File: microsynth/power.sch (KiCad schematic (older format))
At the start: 4 parts, among them J2 AudioJack2, J3 AudioJack2, J4 AudioJack2, J5 AudioJack2

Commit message: Footprints 2
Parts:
- J2, J3, J4, J5: footprint (none) -> Connector_Audio:Jack_3.5mm_QingPu_WQP-PJ398SM_Vertical_CircularHoles
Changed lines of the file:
@@
 F 0 "J2" H 3820 2170 50  0000 R CNN
 F 1 "AudioJack2" H 3820 2079 50  0000 R CNN
-F 2 "" H 4000 2050 50  0001 C CNN
+F 2 "Connector_Audio:Jack_3.5mm_QingPu_WQP-PJ398SM_Vertical_CircularHoles" H 4000 2050 50  0001 C CNN
 F 3 "~" H 4000 2050 50  0001 C CNN
 F 4 "TRIGGER OUT" H 3820 1988 50  0000 R CNN "Label"
@@
 F 0 "J3" H 3820 2620 50  0000 R CNN
 F 1 "AudioJack2" H 3820 2529 50  0000 R CNN
-F 2 "" H 4000 2500 50  0001 C CNN
+F 2 "Connector_Audio:Jack_3.5mm_QingPu_WQP-PJ398SM_Vertical_CircularHoles" H 4000 2500 50  0001 C CNN
 F 3 "~" H 4000 2500 50  0001 C CNN
 F 4 "KEYBOARD VOLTAGE OUT" H 3820 2438 50  0000 R CNN "Label"
@@
 F 0 "J4" H 3820 3070 50  0000 R CNN
 F 1 "AudioJack2" H 3820 2979 50  0000 R CNN
-F 2 "" H 4000 2950 50  0001 C CNN
+F 2 "Connector_Audio:Jack_3.5mm_QingPu_WQP-PJ398SM_Vertical_CircularHoles" H 4000 2950 50  0001 C CNN
 F 3 "~" H 4000 2950 50  0001 C CNN
 F 4 "TRIGGER IN" H 3820 2888 50  0000 R CNN "Label"
@@
 F 0 "J5" H 3820 3520 50  0000 R CNN
 F 1 "AudioJack2" H 3820 3429 50  0000 R CNN
-F 2 "" H 4000 3400 50  0001 C CNN
+F 2 "Connector_Audio:Jack_3.5mm_QingPu_WQP-PJ398SM_Vertical_CircularHoles" H 4000 3400 50  0001 C CNN
 F 3 "~" H 4000 3400 50  0001 C CNN
 F 4 "KEYBOARD VOLTAGE OUT" H 3820 3338 50  0000 R CNN "Label"

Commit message: Hacking together the footprints
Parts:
- J2, J3, J4, J5: footprint Connector_Audio:Jack_3.5mm_QingPu_WQP-PJ398SM_Vertical_CircularHoles -> 4ms_Jack:EighthInch_Stereo_PJ366ST_ALT
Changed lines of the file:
@@
 F 0 "J2" H 3820 2170 50  0000 R CNN
 F 1 "AudioJack2" H 3820 2079 50  0000 R CNN
-F 2 "Connector_Audio:Jack_3.5mm_QingPu_WQP-PJ398SM_Vertical_CircularHoles" H 4000 2050 50  0001 C CNN
+F 2 "4ms_Jack:EighthInch_Stereo_PJ366ST_ALT" H 4000 2050 50  0001 C CNN
 F 3 "~" H 4000 2050 50  0001 C CNN
 F 4 "TRIGGER OUT" H 3820 1988 50  0000 R CNN "Label"
@@
 F 0 "J3" H 3820 2620 50  0000 R CNN
 F 1 "AudioJack2" H 3820 2529 50  0000 R CNN
-F 2 "Connector_Audio:Jack_3.5mm_QingPu_WQP-PJ398SM_Vertical_CircularHoles" H 4000 2500 50  0001 C CNN
+F 2 "4ms_Jack:EighthInch_Stereo_PJ366ST_ALT" H 4000 2500 50  0001 C CNN
 F 3 "~" H 4000 2500 50  0001 C CNN
 F 4 "KEYBOARD VOLTAGE OUT" H 3820 2438 50  0000 R CNN "Label"
@@
 F 0 "J4" H 3820 3070 50  0000 R CNN
 F 1 "AudioJack2" H 3820 2979 50  0000 R CNN
-F 2 "Connector_Audio:Jack_3.5mm_QingPu_WQP-PJ398SM_Vertical_CircularHoles" H 4000 2950 50  0001 C CNN
+F 2 "4ms_Jack:EighthInch_Stereo_PJ366ST_ALT" H 4000 2950 50  0001 C CNN
 F 3 "~" H 4000 2950 50  0001 C CNN
 F 4 "TRIGGER IN" H 3820 2888 50  0000 R CNN "Label"
@@
 F 0 "J5" H 3820 3520 50  0000 R CNN
 F 1 "AudioJack2" H 3820 3429 50  0000 R CNN
-F 2 "Connector_Audio:Jack_3.5mm_QingPu_WQP-PJ398SM_Vertical_CircularHoles" H 4000 3400 50  0001 C CNN
+F 2 "4ms_Jack:EighthInch_Stereo_PJ366ST_ALT" H 4000 3400 50  0001 C CNN
 F 3 "~" H 4000 3400 50  0001 C CNN
 F 4 "KEYBOARD VOLTAGE OUT" H 3820 3338 50  0000 R CNN "Label"

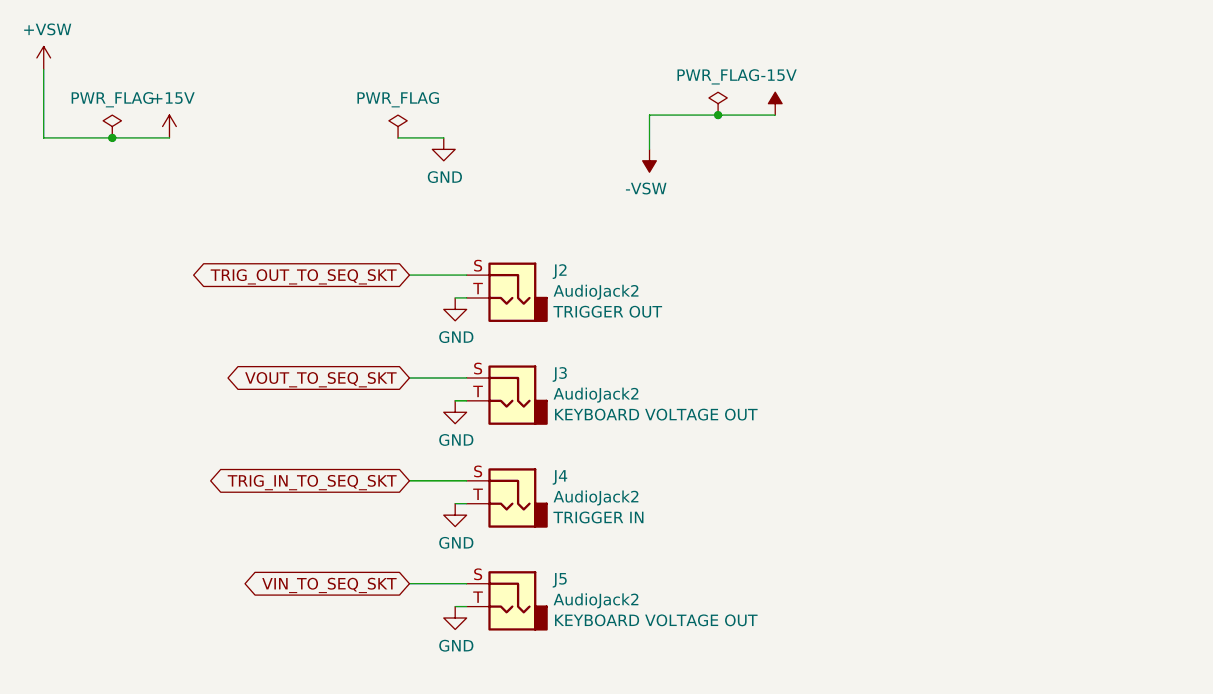
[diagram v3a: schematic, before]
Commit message: Laying out pcb
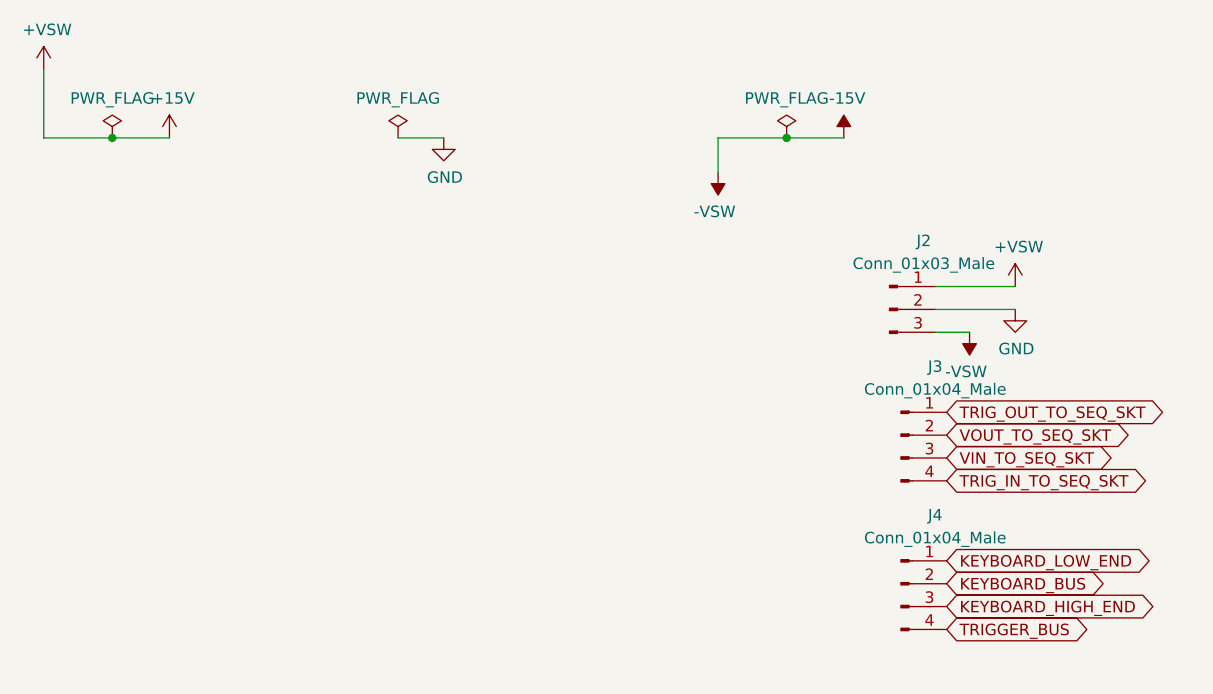
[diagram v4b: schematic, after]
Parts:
- removed J2, J3, J4, J5: AudioJack2, 4ms_Jack:EighthInch_Stereo_PJ366ST_ALT, symbol Connector:AudioJack2
- added J2: Conn_01x03_Male, Connector_PinHeader_2.54mm:PinHeader_1x03_P2.54mm_Horizontal, symbol Connector:Conn_01x03_Male
- added J3, J4: Conn_01x04_Male, Connector_PinHeader_2.54mm:PinHeader_1x04_P2.54mm_Horizontal, symbol Connector:Conn_01x04_Male
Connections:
- net +15V: now also J2.1 (Pin_1)
- net -15V: now also J2.3 (Pin_3)
- net GND: now also J2.2 (Pin_2)
- net TRIG_IN_TO_SEQ_SKT: now also J3.4 (Pin_4)
- net TRIG_OUT_TO_SEQ_SKT: now also J3.1 (Pin_1)
- net VIN_TO_SEQ_SKT: now also J3.3 (Pin_3)
- net VOUT_TO_SEQ_SKT: now also J3.2 (Pin_2)
- new net KEYBOARD_BUS: J4.2 (Pin_2)
- new net KEYBOARD_HIGH_END: J4.3 (Pin_3)
- new net KEYBOARD_LOW_END: J4.1 (Pin_1)
- new net TRIGGER_BUS: J4.4 (Pin_4)
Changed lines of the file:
@@
 L power:-15V #PWR0102
 U 1 1 5E05F00D
-P 5150 1250
-F 0 "#PWR0102" H 5150 1350 50  0001 C CNN
-F 1 "-15V" H 5165 1423 50  0000 C CNN
-F 2 "" H 5150 1250 50  0001 C CNN
-F 3 "" H 5150 1250 50  0001 C CNN
-	1    5150 1250
+P 5450 1350
+F 0 "#PWR0102" H 5450 1450 50  0001 C CNN
+F 1 "-15V" H 5465 1523 50  0000 C CNN
+F 2 "" H 5450 1350 50  0001 C CNN
+F 3 "" H 5450 1350 50  0001 C CNN
+	1    5450 1350
 	1    0    0    -1
 $EndComp
@@
 $EndComp
 Wire Wire Line
-	4600 1250 4900 1250
+	4900 1350 5200 1350
 $Comp
 L power:PWR_FLAG #FLG0102
 U 1 1 5E0610BE
-P 4900 1250
-F 0 "#FLG0102" H 4900 1325 50  0001 C CNN
-F 1 "PWR_FLAG" H 4900 1423 50  0000 C CNN
-F 2 "" H 4900 1250 50  0001 C CNN
-F 3 "~" H 4900 1250 50  0001 C CNN
-	1    4900 1250
+P 5200 1350
+F 0 "#FLG0102" H 5200 1425 50  0001 C CNN
+F 1 "PWR_FLAG" H 5200 1523 50  0000 C CNN
+F 2 "" H 5200 1350 50  0001 C CNN
+F 3 "~" H 5200 1350 50  0001 C CNN
+	1    5200 1350
 	1    0    0    -1
 $EndComp
-Connection ~ 4900 1250
+Connection ~ 5200 1350
 Wire Wire Line
-	4900 1250 5150 1250
+	5200 1350 5450 1350
 $Comp
 L power:PWR_FLAG #FLG0103
@@
 L power:-VSW #PWR0124
 U 1 1 5E201FCA
-P 4600 1400
-F 0 "#PWR0124" H 4600 1500 50  0001 C CNN
-F 1 "-VSW" H 4615 1573 50  0000 C CNN
-F 2 "" H 4600 1400 50  0001 C CNN
-F 3 "" H 4600 1400 50  0001 C CNN
-	1    4600 1400
+P 4900 1500
+F 0 "#PWR0124" H 4900 1600 50  0001 C CNN
+F 1 "-VSW" H 4915 1673 50  0000 C CNN
+F 2 "" H 4900 1500 50  0001 C CNN
+F 3 "" H 4900 1500 50  0001 C CNN
+	1    4900 1500
 	-1   0    0    1
 $EndComp
 Wire Wire Line
-	4600 1400 4600 1250
-$Comp
-L Connector:AudioJack2 J2
-U 1 1 5EFEF0E1
-P 4000 2050
-F 0 "J2" H 3820 2170 50  0000 R CNN
-F 1 "AudioJack2" H 3820 2079 50  0000 R CNN
-F 2 "4ms_Jack:EighthInch_Stereo_PJ366ST_ALT" H 4000 2050 50  0001 C CNN
-F 3 "~" H 4000 2050 50  0001 C CNN
-F 4 "TRIGGER OUT" H 3820 1988 50  0000 R CNN "Label"
-	1    4000 2050
-	-1   0    0    -1
-$EndComp
-$Comp
-L power:GND #PWR0228
-U 1 1 5EFEFF0A
-P 3750 2050
-F 0 "#PWR0228" H 3750 1800 50  0001 C CNN
-F 1 "GND" H 3755 1877 50  0000 C CNN
-F 2 "" H 3750 2050 50  0001 C CNN
-F 3 "" H 3750 2050 50  0001 C CNN
-	1    3750 2050
-	1    0    0    -1
-$EndComp
-Wire Wire Line
-	3750 2050 3800 2050
-$Comp
-L Connector:AudioJack2 J3
-U 1 1 5EFF0BC3
-P 4000 2500
-F 0 "J3" H 3820 2620 50  0000 R CNN
-F 1 "AudioJack2" H 3820 2529 50  0000 R CNN
-F 2 "4ms_Jack:EighthInch_Stereo_PJ366ST_ALT" H 4000 2500 50  0001 C CNN
-F 3 "~" H 4000 2500 50  0001 C CNN
-F 4 "KEYBOARD VOLTAGE OUT" H 3820 2438 50  0000 R CNN "Label"
-	1    4000 2500
-	-1   0    0    -1
-$EndComp
-$Comp
-L power:GND #PWR0229
-U 1 1 5EFF0BC9
-P 3750 2500
-F 0 "#PWR0229" H 3750 2250 50  0001 C CNN
-F 1 "GND" H 3755 2327 50  0000 C CNN
-F 2 "" H 3750 2500 50  0001 C CNN
-F 3 "" H 3750 2500 50  0001 C CNN
-	1    3750 2500
-	1    0    0    -1
-$EndComp
-Wire Wire Line
-	3750 2500 3800 2500
-$Comp
-L Connector:AudioJack2 J4
-U 1 1 5EFF1653
-P 4000 2950
-F 0 "J4" H 3820 3070 50  0000 R CNN
-F 1 "AudioJack2" H 3820 2979 50  0000 R CNN
-F 2 "4ms_Jack:EighthInch_Stereo_PJ366ST_ALT" H 4000 2950 50  0001 C CNN
-F 3 "~" H 4000 2950 50  0001 C CNN
-F 4 "TRIGGER IN" H 3820 2888 50  0000 R CNN "Label"
-	1    4000 2950
-	-1   0    0    -1
-$EndComp
-$Comp
-L power:GND #PWR0230
-U 1 1 5EFF1659
-P 3750 2950
-F 0 "#PWR0230" H 3750 2700 50  0001 C CNN
-F 1 "GND" H 3755 2777 50  0000 C CNN
-F 2 "" H 3750 2950 50  0001 C CNN
-F 3 "" H 3750 2950 50  0001 C CNN
-	1    3750 2950
-	1    0    0    -1
-$EndComp
-Wire Wire Line
-	3750 2950 3800 2950
-$Comp
-L Connector:AudioJack2 J5
-U 1 1 5EFF23EA
-P 4000 3400
-F 0 "J5" H 3820 3520 50  0000 R CNN
-F 1 "AudioJack2" H 3820 3429 50  0000 R CNN
-F 2 "4ms_Jack:EighthInch_Stereo_PJ366ST_ALT" H 4000 3400 50  0001 C CNN
-F 3 "~" H 4000 3400 50  0001 C CNN
-F 4 "KEYBOARD VOLTAGE OUT" H 3820 3338 50  0000 R CNN "Label"
-	1    4000 3400
-	-1   0    0    -1
-$EndComp
-$Comp
-L power:GND #PWR0231
-U 1 1 5EFF23F0
-P 3750 3400
-F 0 "#PWR0231" H 3750 3150 50  0001 C CNN
-F 1 "GND" H 3755 3227 50  0000 C CNN
-F 2 "" H 3750 3400 50  0001 C CNN
-F 3 "" H 3750 3400 50  0001 C CNN
-	1    3750 3400
-	1    0    0    -1
-$EndComp
-Wire Wire Line
-	3750 3400 3800 3400
-Text GLabel 3550 2850 0    50   BiDi ~ 0
+	4900 1500 4900 1350
+Text GLabel 5900 2850 2    50   BiDi ~ 0
 TRIG_IN_TO_SEQ_SKT
-Wire Wire Line
-	3550 2850 3800 2850
-Text GLabel 3550 2400 0    50   BiDi ~ 0
+Text GLabel 5900 2650 2    50   BiDi ~ 0
 VOUT_TO_SEQ_SKT
-Wire Wire Line
-	3550 2400 3800 2400
-Text GLabel 3550 3300 0    50   BiDi ~ 0
+Text GLabel 5900 2750 2    50   BiDi ~ 0
 VIN_TO_SEQ_SKT
-Wire Wire Line
-	3550 3300 3800 3300
-Text GLabel 3550 1950 0    50   BiDi ~ 0
+Text GLabel 5900 2550 2    50   BiDi ~ 0
 TRIG_OUT_TO_SEQ_SKT
-Wire Wire Line
-	3550 1950 3800 1950
 Connection ~ 2250 1350
 Wire Wire Line
@@
 Wire Wire Line
 	1950 1350 2250 1350
+$Comp
+L Connector:Conn_01x03_Male J2
+U 1 1 5F1FC317
+P 5650 2100
+F 0 "J2" H 5800 2400 50  0000 C CNN
+F 1 "Conn_01x03_Male" H 5800 2300 50  0000 C CNN
+F 2 "Connector_PinHeader_2.54mm:PinHeader_1x03_P2.54mm_Horizontal" H 5650 2100 50  0001 C CNN
+F 3 "~" H 5650 2100 50  0001 C CNN
+	1    5650 2100
+	1    0    0    -1
+$EndComp
+$Comp
+L Connector:Conn_01x04_Male J3
+U 1 1 5F1FD92E
+P 5700 2650
+F 0 "J3" H 5850 2950 50  0000 C CNN
+F 1 "Conn_01x04_Male" H 5850 2850 50  0000 C CNN
+F 2 "Connector_PinHeader_2.54mm:PinHeader_1x04_P2.54mm_Horizontal" H 5700 2650 50  0001 C CNN
+F 3 "~" H 5700 2650 50  0001 C CNN
+	1    5700 2650
+	1    0    0    -1
+$EndComp
+$Comp
+L Connector:Conn_01x04_Male J4
+U 1 1 5F1FE242
+P 5700 3300
+F 0 "J4" H 5850 3600 50  0000 C CNN
+F 1 "Conn_01x04_Male" H 5850 3500 50  0000 C CNN
+F 2 "Connector_PinHeader_2.54mm:PinHeader_1x04_P2.54mm_Horizontal" H 5700 3300 50  0001 C CNN
+F 3 "~" H 5700 3300 50  0001 C CNN
+	1    5700 3300
+	1    0    0    -1
+$EndComp
+Text GLabel 5900 3400 2    50   BiDi ~ 0
+KEYBOARD_HIGH_END
+Text GLabel 5900 3200 2    50   BiDi ~ 0
+KEYBOARD_LOW_END
+Text GLabel 5900 3300 2    50   BiDi ~ 0
+KEYBOARD_BUS
+Text GLabel 5900 3500 2    50   BiDi ~ 0
+TRIGGER_BUS
+$Comp
+L power:-VSW #PWR02
+U 1 1 5F231D96
+P 6000 2200
+F 0 "#PWR02" H 6000 2300 50  0001 C CNN
+F 1 "-VSW" H 6015 2373 50  0000 C CNN
+F 2 "" H 6000 2200 50  0001 C CNN
+F 3 "" H 6000 2200 50  0001 C CNN
+	1    6000 2200
+	-1   0    0    1
+$EndComp
+Wire Wire Line
+	5850 2200 6000 2200
+$Comp
+L power:GND #PWR04
+U 1 1 5F232962
+P 6200 2100
+F 0 "#PWR04" H 6200 1850 50  0001 C CNN
+F 1 "GND" H 6205 1927 50  0000 C CNN
+F 2 "" H 6200 2100 50  0001 C CNN
+F 3 "" H 6200 2100 50  0001 C CNN
+	1    6200 2100
+	1    0    0    -1
+$EndComp
+Wire Wire Line
+	6200 2100 5850 2100
+$Comp
+L power:+VSW #PWR03
+U 1 1 5F233149
+P 6200 2000
+F 0 "#PWR03" H 6200 1850 50  0001 C CNN
+F 1 "+VSW" H 6215 2173 50  0000 C CNN
+F 2 "" H 6200 2000 50  0001 C CNN
+F 3 "" H 6200 2000 50  0001 C CNN
+	1    6200 2000
+	1    0    0    -1
+$EndComp
+Wire Wire Line
+	6200 2000 5850 2000
 $EndSCHEMATC

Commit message: Layout...
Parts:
- J3, J4: footprint Connector_PinHeader_2.54mm:PinHeader_1x04_P2.54mm_Horizontal -> Connector_PinHeader_2.54mm:PinHeader_1x04_P2.54mm_Vertical
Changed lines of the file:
@@
 F 0 "J3" H 5850 2950 50  0000 C CNN
 F 1 "Conn_01x04_Male" H 5850 2850 50  0000 C CNN
-F 2 "Connector_PinHeader_2.54mm:PinHeader_1x04_P2.54mm_Horizontal" H 5700 2650 50  0001 C CNN
+F 2 "Connector_PinHeader_2.54mm:PinHeader_1x04_P2.54mm_Vertical" H 5700 2650 50  0001 C CNN
 F 3 "~" H 5700 2650 50  0001 C CNN
 	1    5700 2650
@@
 F 0 "J4" H 5850 3600 50  0000 C CNN
 F 1 "Conn_01x04_Male" H 5850 3500 50  0000 C CNN
-F 2 "Connector_PinHeader_2.54mm:PinHeader_1x04_P2.54mm_Horizontal" H 5700 3300 50  0001 C CNN
+F 2 "Connector_PinHeader_2.54mm:PinHeader_1x04_P2.54mm_Vertical" H 5700 3300 50  0001 C CNN
 F 3 "~" H 5700 3300 50  0001 C CNN
 	1    5700 3300

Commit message: Tidy up, name switches, proper footprints for all trimmers
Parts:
- J2: footprint Connector_PinHeader_2.54mm:PinHeader_1x03_P2.54mm_Horizontal -> Connector_PinHeader_2.54mm:PinHeader_1x03_P2.54mm_Vertical
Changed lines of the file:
@@
 F 0 "J2" H 5800 2400 50  0000 C CNN
 F 1 "Conn_01x03_Male" H 5800 2300 50  0000 C CNN
-F 2 "Connector_PinHeader_2.54mm:PinHeader_1x03_P2.54mm_Horizontal" H 5650 2100 50  0001 C CNN
+F 2 "Connector_PinHeader_2.54mm:PinHeader_1x03_P2.54mm_Vertical" H 5650 2100 50  0001 C CNN
 F 3 "~" H 5650 2100 50  0001 C CNN
 	1    5650 2100

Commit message: Add new V input
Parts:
- J3: footprint Connector_PinHeader_2.54mm:PinHeader_1x04_P2.54mm_Vertical -> Connector_PinHeader_2.54mm:PinHeader_1x05_P2.54mm_Vertical; symbol Connector:Conn_01x04_Male -> Connector:Conn_01x05_Male
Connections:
- new net VIN_FROM_SEQ: J3.5 (Pin_5)
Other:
- moved on the sheet: J4
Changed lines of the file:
@@
 Wire Wire Line
 	4900 1500 4900 1350
-Text GLabel 5900 2850 2    50   BiDi ~ 0
+Text GLabel 5900 2900 2    50   BiDi ~ 0
 TRIG_IN_TO_SEQ_SKT
-Text GLabel 5900 2650 2    50   BiDi ~ 0
+Text GLabel 5900 2700 2    50   BiDi ~ 0
 VOUT_TO_SEQ_SKT
-Text GLabel 5900 2750 2    50   BiDi ~ 0
+Text GLabel 5900 2800 2    50   BiDi ~ 0
 VIN_TO_SEQ_SKT
-Text GLabel 5900 2550 2    50   BiDi ~ 0
+Text GLabel 5900 2600 2    50   BiDi ~ 0
 TRIG_OUT_TO_SEQ_SKT
 Connection ~ 2250 1350
@@
 $EndComp
 $Comp
-L Connector:Conn_01x04_Male J3
+L Connector:Conn_01x05_Male J3
 U 1 1 5F1FD92E
-P 5700 2650
-F 0 "J3" H 5850 2950 50  0000 C CNN
-F 1 "Conn_01x04_Male" H 5850 2850 50  0000 C CNN
-F 2 "Connector_PinHeader_2.54mm:PinHeader_1x04_P2.54mm_Vertical" H 5700 2650 50  0001 C CNN
-F 3 "~" H 5700 2650 50  0001 C CNN
-	1    5700 2650
+P 5700 2800
+F 0 "J3" H 5700 3200 50  0000 C CNN
+F 1 "Conn_01x04_Male" H 6000 3100 50  0000 C CNN
+F 2 "Connector_PinHeader_2.54mm:PinHeader_1x05_P2.54mm_Vertical" H 5700 2800 50  0001 C CNN
+F 3 "~" H 5700 2800 50  0001 C CNN
+	1    5700 2800
 	1    0    0    -1
 $EndComp
@@
 L Connector:Conn_01x04_Male J4
 U 1 1 5F1FE242
-P 5700 3300
-F 0 "J4" H 5850 3600 50  0000 C CNN
-F 1 "Conn_01x04_Male" H 5850 3500 50  0000 C CNN
-F 2 "Connector_PinHeader_2.54mm:PinHeader_1x04_P2.54mm_Vertical" H 5700 3300 50  0001 C CNN
-F 3 "~" H 5700 3300 50  0001 C CNN
-	1    5700 3300
+P 5700 3450
+F 0 "J4" H 5850 3750 50  0000 C CNN
+F 1 "Conn_01x04_Male" H 5850 3650 50  0000 C CNN
+F 2 "Connector_PinHeader_2.54mm:PinHeader_1x04_P2.54mm_Vertical" H 5700 3450 50  0001 C CNN
+F 3 "~" H 5700 3450 50  0001 C CNN
+	1    5700 3450
 	1    0    0    -1
 $EndComp
-Text GLabel 5900 3400 2    50   BiDi ~ 0
+Text GLabel 5900 3550 2    50   BiDi ~ 0
 KEYBOARD_HIGH_END
-Text GLabel 5900 3200 2    50   BiDi ~ 0
+Text GLabel 5900 3350 2    50   BiDi ~ 0
 KEYBOARD_LOW_END
-Text GLabel 5900 3300 2    50   BiDi ~ 0
+Text GLabel 5900 3450 2    50   BiDi ~ 0
 KEYBOARD_BUS
-Text GLabel 5900 3500 2    50   BiDi ~ 0
+Text GLabel 5900 3650 2    50   BiDi ~ 0
 TRIGGER_BUS
 $Comp
@@
 Wire Wire Line
 	6200 2000 5850 2000
+Text GLabel 5900 3000 2    50   Input ~ 0
+VIN_FROM_SEQ
 $EndSCHEMATC
